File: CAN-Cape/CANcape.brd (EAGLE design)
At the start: 58.4 x 77.5 mm, 9 parts

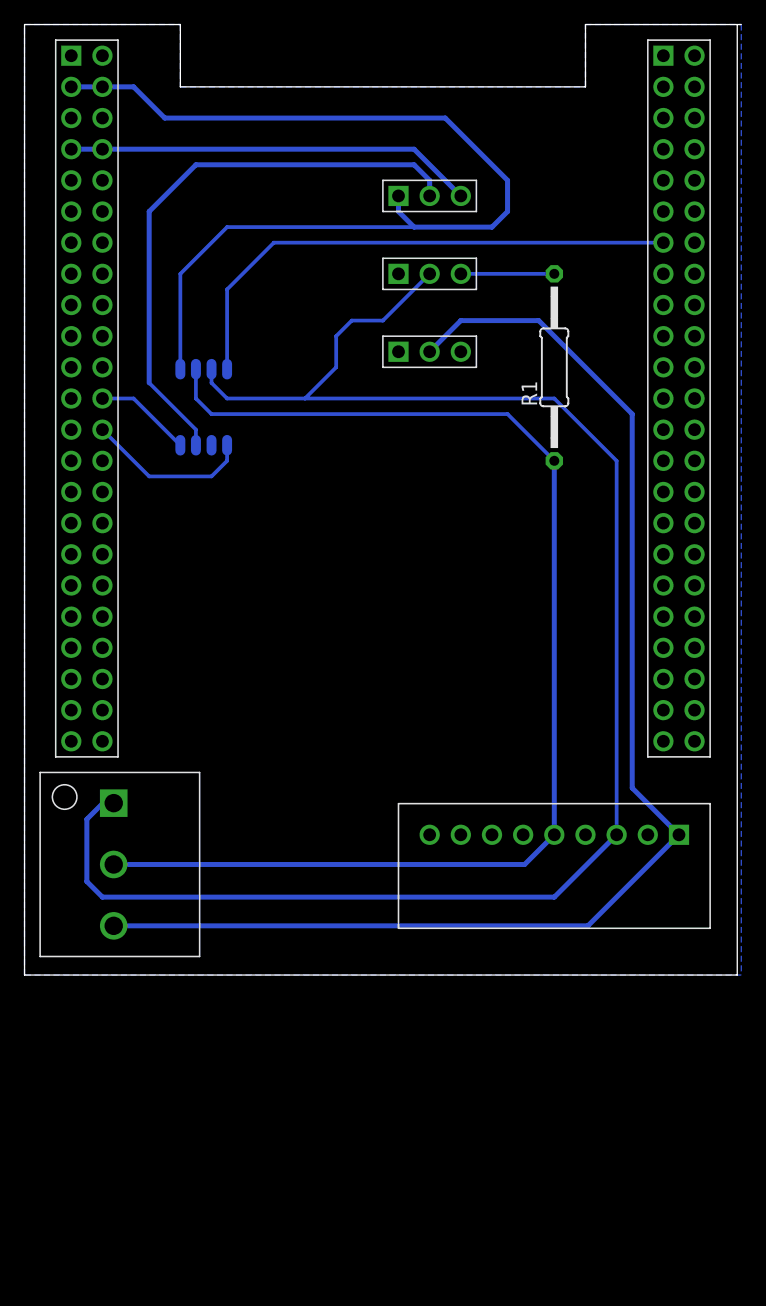
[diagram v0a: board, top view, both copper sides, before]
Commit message: more board work
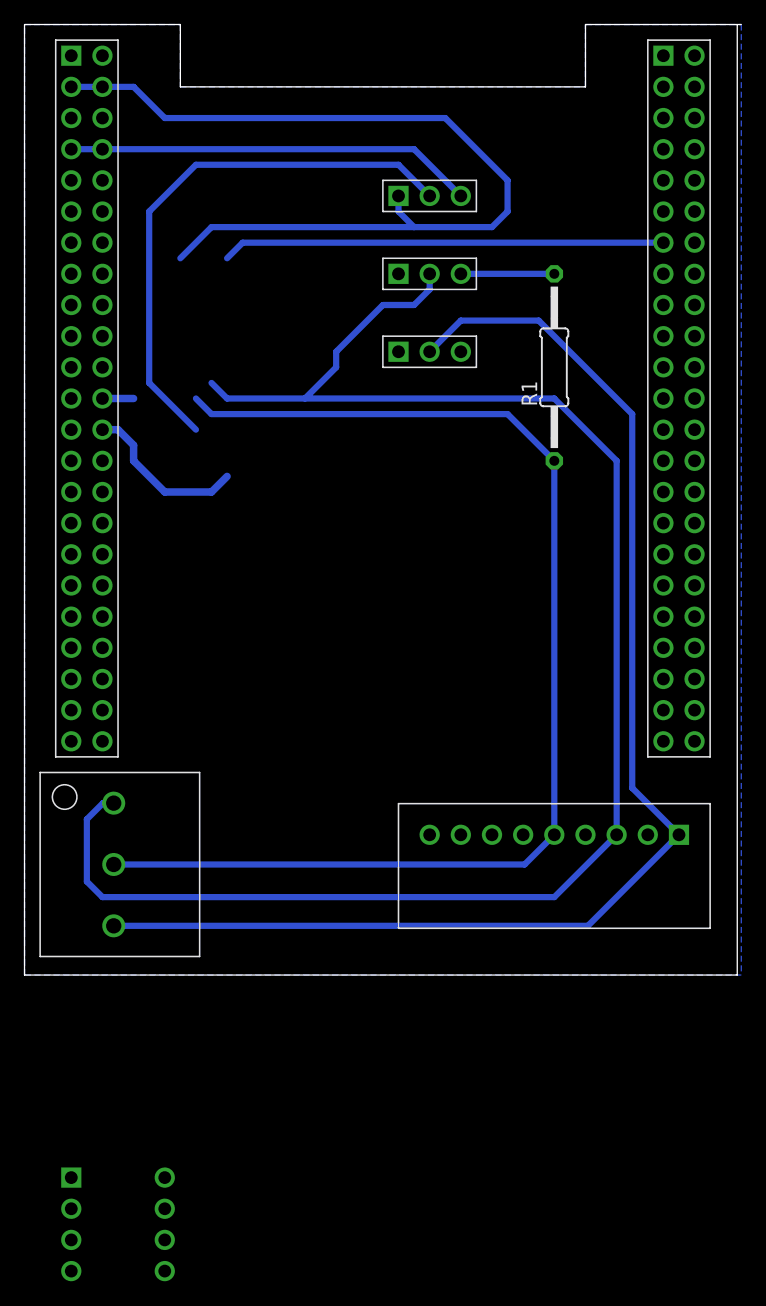
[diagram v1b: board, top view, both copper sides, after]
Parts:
- U$5: value SN65HVD320 -> SOIC_BREAKOUT; device SPST-switch:SN65HVD320 -> CANcape:SOIC_BREAKOUT
- moved U$5 64.1 mm to (8.89, -21.6), flipped to the top
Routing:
- net 3.3V: track 80.9 -> 72.6 mm
- net STANDBY: track 43.6 -> 36.1 mm
- net DCAN1_RX: track 7.93 -> 2.54 mm
- net CANL: track 101.1 -> 98.7 mm
- net TRAN_PWR: track 46.9 -> 44.8 mm
- net CANH: track 136.7 -> 135.6 mm
